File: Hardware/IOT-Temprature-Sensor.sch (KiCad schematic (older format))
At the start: 48 parts, among them IC3 NST1001, J1 Conn_01x04_Male, Q1 CJE3139K, Q2 MMBT3904, Q3 MMBT3904, SW1 SW_1003B, SW2 SW_1003B, U1 OPL1200, Y1 32.768KHZ, Y4 22MHZ

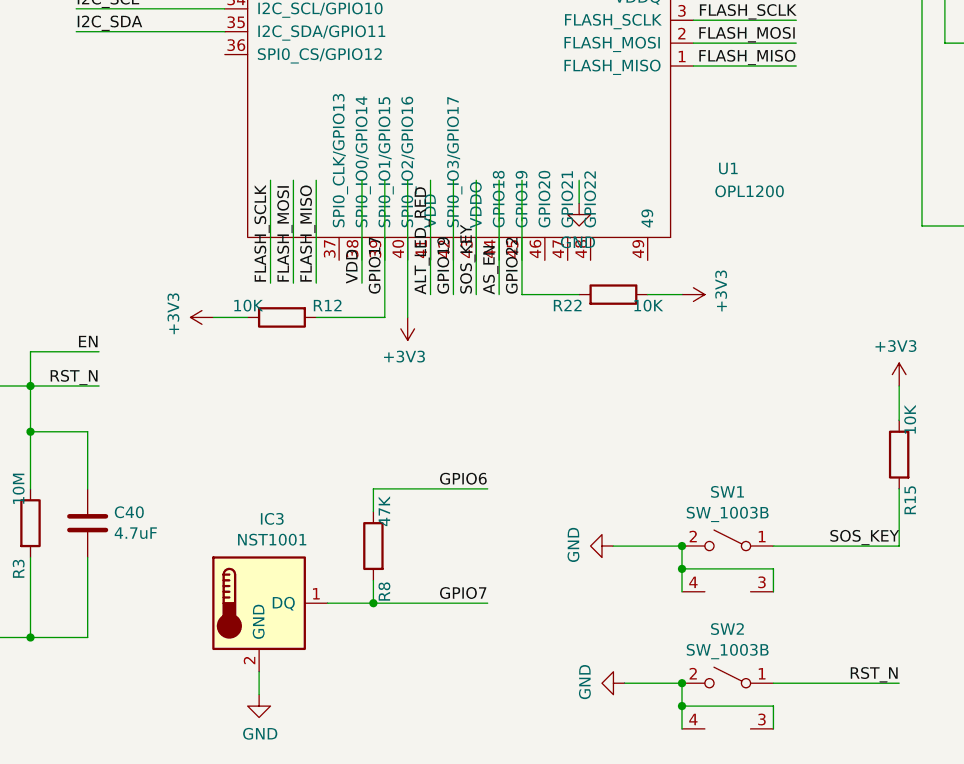
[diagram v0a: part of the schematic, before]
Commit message: xiaoming-opensource
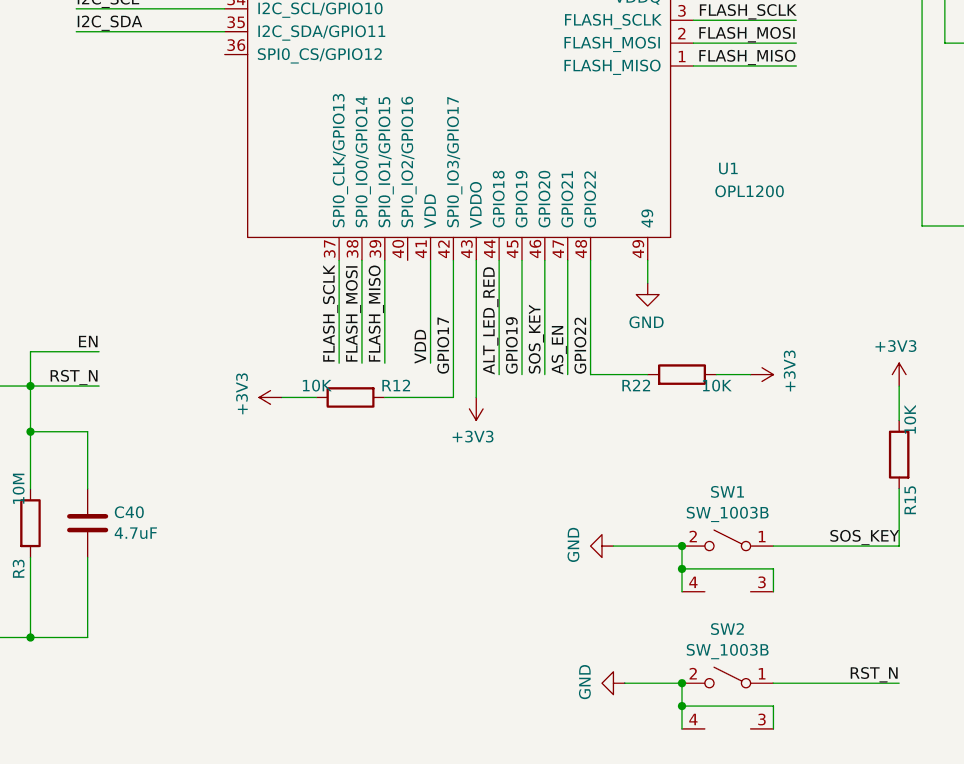
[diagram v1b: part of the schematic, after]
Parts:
- removed IC3: NST1001, Sensor_Voltage:NST1001NEW, symbol Medical_Ring-v5.2-rescue:NST1001-Sensor_Temperature
- removed R8: 47K, Resistor_SMD:R_0402_1005Metric, symbol Medical_Ring-v5.2-rescue:R-Device
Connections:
- wire segments 202 -> 196
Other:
- moved on the sheet: R12, R22
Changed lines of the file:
@@
 	5050 4450 5500 4450
 Wire Wire Line
-	3400 5150 3400 5600
-Text Label 3400 5600 1    50   ~ 0
+	3700 5500 3700 5950
+Text Label 3700 5950 1    50   ~ 0
 FLASH_MISO
-Text Label 3300 5600 1    50   ~ 0
+Text Label 3600 5950 1    50   ~ 0
 FLASH_MOSI
-Text Label 3200 5600 1    50   ~ 0
+Text Label 3500 5950 1    50   ~ 0
 FLASH_SCLK
 Wire Wire Line
-	3300 5150 3300 5600
-Wire Wire Line
-	3200 5150 3200 5600
+	3600 5500 3600 5950
+Wire Wire Line
+	3500 5500 3500 5950
 Wire Wire Line
 	3000 3900 1500 3900
@@
 VDD_RF
 Wire Wire Line
-	3600 5150 3600 5600
-Text Label 3600 5450 3    50   ~ 0
+	3900 5500 3900 5950
+Text Label 3900 5800 3    50   ~ 0
 VDD
 $Comp
 L Medical_Ring-v5.2-rescue:GND-power #PWR0104
 U 1 1 5EC08210
-P 4550 5250
+P 4850 5600
 AR Path="/5EC08210" Ref="#PWR0104"  Part="1"
 AR Path="/5EB63113/5EC08210" Ref="#PWR0159"  Part="1"
 AR Path="/6180F478/5EC08210" Ref="#PWR?"  Part="1"
-F 0 "#PWR0104" H 4550 5000 50  0001 C CNN
-F 1 "GND" H 4555 5077 50  0000 C CNN
-F 2 "" H 4550 5250 50  0001 C CNN
-F 3 "" H 4550 5250 50  0001 C CNN
-	1    4550 5250
+F 0 "#PWR0104" H 4850 5350 50  0001 C CNN
+F 1 "GND" H 4855 5427 50  0000 C CNN
+F 2 "" H 4850 5600 50  0001 C CNN
+F 3 "" H 4850 5600 50  0001 C CNN
+	1    4850 5600
 	-1   0    0    -1
 $EndComp
 Wire Wire Line
-	4550 5150 4550 5250
+	4850 5500 4850 5600
 Text Label 3800 2050 3    50   ~ 0
 VDD
@@
 Wire Wire Line
 	4200 1350 4200 1500
-Text Label 4300 5650 1    50   ~ 0
+Text Label 4600 6000 1    50   ~ 0
 GPIO22
 Wire Wire Line
@@
 L Medical_Ring-v5.2-rescue:+3V3-power #PWR0122
 U 1 1 5EEC6474
-P 3800 5750
-F 0 "#PWR0122" H 3800 5600 50  0001 C CNN
-F 1 "+3V3" H 3815 5923 50  0000 C CNN
-F 2 "" H 3800 5750 50  0001 C CNN
-F 3 "" H 3800 5750 50  0001 C CNN
-	1    3800 5750
+P 4100 6100
+F 0 "#PWR0122" H 4100 5950 50  0001 C CNN
+F 1 "+3V3" H 4115 6273 50  0000 C CNN
+F 2 "" H 4100 6100 50  0001 C CNN
+F 3 "" H 4100 6100 50  0001 C CNN
+	1    4100 6100
 	-1   0    0    1
 $EndComp
@@
 Text Label 2500 4000 0    50   ~ 0
 ALT_LED
-Text Label 4100 5650 1    50   ~ 0
+Text Label 4400 6000 1    50   ~ 0
 SOS_KEY
 $Comp
@@
 	0    -1   -1   0
 $EndComp
-Text Label 4200 5650 1    50   ~ 0
+Text Label 4500 6000 1    50   ~ 0
 AS_EN
 Wire Wire Line
@@
 AS_EN
 Wire Wire Line
-	4200 5150 4200 5650
+	4500 5500 4500 6000
 Wire Wire Line
 	8850 4350 8350 4350
@@
 Text Label 8350 2150 0    50   ~ 0
 ALT_LED_RED
-Text Label 3900 5650 1    50   ~ 0
+Text Label 4200 6000 1    50   ~ 0
 ALT_LED_RED
 $Comp
@@
 $EndComp
 Wire Wire Line
-	4300 5150 4300 5650
+	4600 5500 4600 6000
 Wire Wire Line
 	3000 3600 2500 3600
@@
 Wire Wire Line
 	8350 4050 8850 4050
-Text Label 3700 5650 1    50   ~ 0
+Text Label 4000 6000 1    50   ~ 0
 GPIO17
 $Comp
@@
 	1750 2050 3700 2050
 Wire Wire Line
-	4100 5150 4100 5650
+	4400 5500 4400 6000
 Wire Wire Line
 	1800 6050 2150 6050
@@
 L Medical_Ring-v5.2-rescue:R-Device R?
 U 1 1 60763174
-P 4700 5650
+P 5000 6000
 AR Path="/5BD78552/60763174" Ref="R?"  Part="1"
 AR Path="/60763174" Ref="R22"  Part="1"
 AR Path="/5EB63113/60763174" Ref="R?"  Part="1"
 AR Path="/6180F478/60763174" Ref="R?"  Part="1"
-F 0 "R22" V 4650 5450 50  0000 C CNN
-F 1 "10K" V 4650 5800 50  0000 C CNN
-F 2 "Resistor_SMD:R_0402_1005Metric" V 4630 5650 50  0001 C CNN
-F 3 "~" H 4700 5650 50  0001 C CNN
-	1    4700 5650
+F 0 "R22" V 4950 5800 50  0000 C CNN
+F 1 "10K" V 4950 6150 50  0000 C CNN
+F 2 "Resistor_SMD:R_0402_1005Metric" V 4930 6000 50  0001 C CNN
+F 3 "~" H 5000 6000 50  0001 C CNN
+	1    5000 6000
 	0    1    -1   0
 $EndComp
 Wire Wire Line
-	4850 5650 5000 5650
+	5150 6000 5300 6000
 $Comp
 L Medical_Ring-v5.2-rescue:+3V3-power #PWR0157
 U 1 1 6076317B
-P 5000 5650
-F 0 "#PWR0157" H 5000 5500 50  0001 C CNN
-F 1 "+3V3" H 5015 5823 50  0000 C CNN
-F 2 "" H 5000 5650 50  0001 C CNN
-F 3 "" H 5000 5650 50  0001 C CNN
-	1    5000 5650
+P 5300 6000
+F 0 "#PWR0157" H 5300 5850 50  0001 C CNN
+F 1 "+3V3" H 5315 6173 50  0000 C CNN
+F 2 "" H 5300 6000 50  0001 C CNN
+F 3 "" H 5300 6000 50  0001 C CNN
+	1    5300 6000
 	0    1    -1   0
 $EndComp
 Wire Wire Line
-	4550 5650 4300 5650
+	4850 6000 4600 6000
 $Comp
 L Medical_Ring-v5.2-rescue:Conn_01x04_Male-Connector J1
@@
 Wire Wire Line
 	3000 4100 2500 4100
-Text Label 4000 5650 1    50   ~ 0
+Text Label 4300 6000 1    50   ~ 0
 GPIO19
 $Sheet
@@
 Connection ~ 1800 2250
 Wire Wire Line
-	3900 5150 3900 5650
-Wire Wire Line
-	4000 5150 4000 5650
+	4200 5500 4200 6000
+Wire Wire Line
+	4300 5500 4300 6000
 $Comp
 L Medical_Ring-v5.2-rescue:SW_1003B-Switch SW1
@@
 L Medical_Ring-v5.2-rescue:R-Device R?
 U 1 1 611E2C38
-P 3250 5750
+P 3550 6100
 AR Path="/5BD78552/611E2C38" Ref="R?"  Part="1"
 AR Path="/611E2C38" Ref="R12"  Part="1"
 AR Path="/5EB63113/611E2C38" Ref="R?"  Part="1"
 AR Path="/6180F478/611E2C38" Ref="R?"  Part="1"
-F 0 "R12" V 3200 5550 50  0000 C CNN
-F 1 "10K" V 3200 5900 50  0000 C CNN
-F 2 "Resistor_SMD:R_0402_1005Metric" V 3180 5750 50  0001 C CNN
-F 3 "~" H 3250 5750 50  0001 C CNN
-	1    3250 5750
+F 0 "R12" V 3500 5900 50  0000 C CNN
+F 1 "10K" V 3500 6250 50  0000 C CNN
+F 2 "Resistor_SMD:R_0402_1005Metric" V 3480 6100 50  0001 C CNN
+F 3 "~" H 3550 6100 50  0001 C CNN
+	1    3550 6100
 	0    -1   1    0
 $EndComp
 Wire Wire Line
-	3100 5750 2950 5750
-Wire Wire Line
-	3800 5150 3800 5750
-Wire Wire Line
-	3700 5150 3700 5750
-Wire Wire Line
-	3400 5750 3700 5750
+	3400 6100 3250 6100
+Wire Wire Line
+	4100 5500 4100 6100
+Wire Wire Line
+	4000 5500 4000 6100
+Wire Wire Line
+	3700 6100 4000 6100
 Text Label 10450 3350 2    50   ~ 0
 GPIO19
@@
 L Medical_Ring-v5.2-rescue:+3V3-power #PWR0102
 U 1 1 61795CF2
-P 2950 5750
+P 3250 6100
 AR Path="/61795CF2" Ref="#PWR0102"  Part="1"
 AR Path="/5EFAEE47/61795CF2" Ref="#PWR?"  Part="1"
 AR Path="/6180F478/61795CF2" Ref="#PWR?"  Part="1"
-F 0 "#PWR0102" H 2950 5600 50  0001 C CNN
-F 1 "+3V3" H 2965 5923 50  0000 C CNN
-F 2 "" H 2950 5750 50  0001 C CNN
-F 3 "" H 2950 5750 50  0001 C CNN
-	1    2950 5750
+F 0 "#PWR0102" H 3250 5950 50  0001 C CNN
+F 1 "+3V3" H 3265 6273 50  0000 C CNN
+F 2 "" H 3250 6100 50  0001 C CNN
+F 3 "" H 3250 6100 50  0001 C CNN
+	1    3250 6100
 	0    -1   -1   0
 $EndComp
 Connection ~ 5000 6750
 Connection ~ 5000 7350
-Text Label 4150 6500 2    50   ~ 0
-GPIO6
-Wire Wire Line
-	3650 6900 3650 7000
-Text Label 4150 7000 2    50   ~ 0
-GPIO7
-Wire Wire Line
-	3650 7000 4150 7000
-Wire Wire Line
-	3650 6500 4150 6500
-Connection ~ 3650 7000
-Wire Wire Line
-	3450 7000 3650 7000
-Wire Wire Line
-	3650 6600 3650 6500
-$Comp
-L Medical_Ring-v5.2-rescue:R-Device R?
-U 1 1 611B3953
-P 3650 6750
-AR Path="/5BD78552/611B3953" Ref="R?"  Part="1"
-AR Path="/611B3953" Ref="R8"  Part="1"
-AR Path="/5EB63113/611B3953" Ref="R?"  Part="1"
-AR Path="/6180F478/611B3953" Ref="R?"  Part="1"
-F 0 "R8" V 3600 6550 50  0000 C CNN
-F 1 "47K" V 3600 6900 50  0000 C CNN
-F 2 "Resistor_SMD:R_0402_1005Metric" V 3580 6750 50  0001 C CNN
-F 3 "~" H 3650 6750 50  0001 C CNN
-	1    3650 6750
-	-1   0    0    -1
-$EndComp
-Wire Wire Line
-	3150 7300 3150 7400
-$Comp
-L Medical_Ring-v5.2-rescue:GND-power #PWR0120
-U 1 1 61195C78
-P 3150 7400
-F 0 "#PWR0120" H 3150 7150 50  0001 C CNN
-F 1 "GND" H 3155 7227 50  0000 C CNN
-F 2 "" H 3150 7400 50  0001 C CNN
-F 3 "" H 3150 7400 50  0001 C CNN
-	1    3150 7400
-	1    0    0    -1
-$EndComp
-$Comp
-L Medical_Ring-v5.2-rescue:NST1001-Sensor_Temperature IC3
-U 1 1 611955C2
-P 3150 7000
-F 0 "IC3" H 3207 7367 50  0000 C CNN
-F 1 "NST1001" H 3207 7276 50  0000 C CNN
-F 2 "Sensor_Voltage:NST1001NEW" H 2150 6750 50  0001 C CNN
-F 3 "http://datasheets.maximintegrated.com/en/ds/MAX31820.pdf" H 3000 7250 50  0001 C CNN
-	1    3150 7000
-	1    0    0    -1
-$EndComp
 $Comp
 L jwatch-rescue:OPL1200-MCU_Module U1
